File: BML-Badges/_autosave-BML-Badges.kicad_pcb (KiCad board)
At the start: 2 copper layers, 19 parts, among them Q1 PN2222A, Q2 PN2222A, Q3 PN2222A

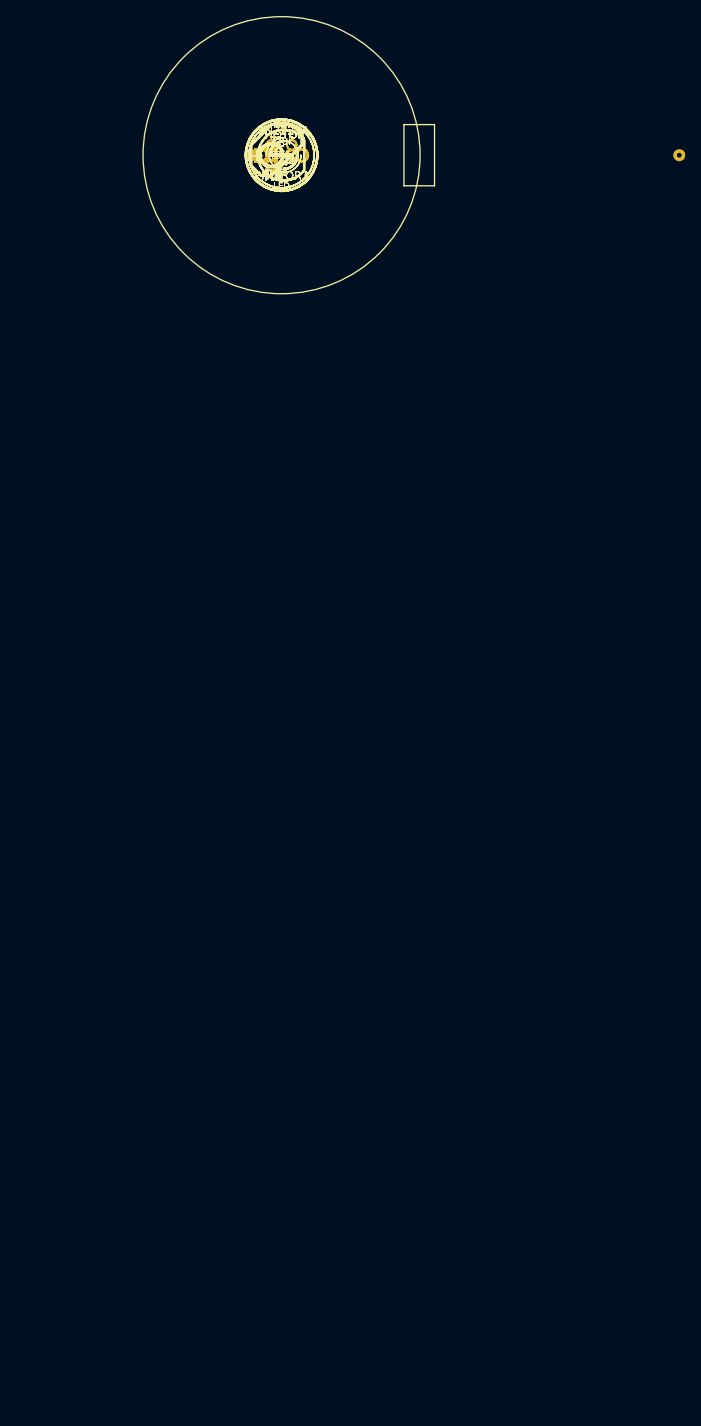
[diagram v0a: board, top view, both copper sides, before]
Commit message: Naptime
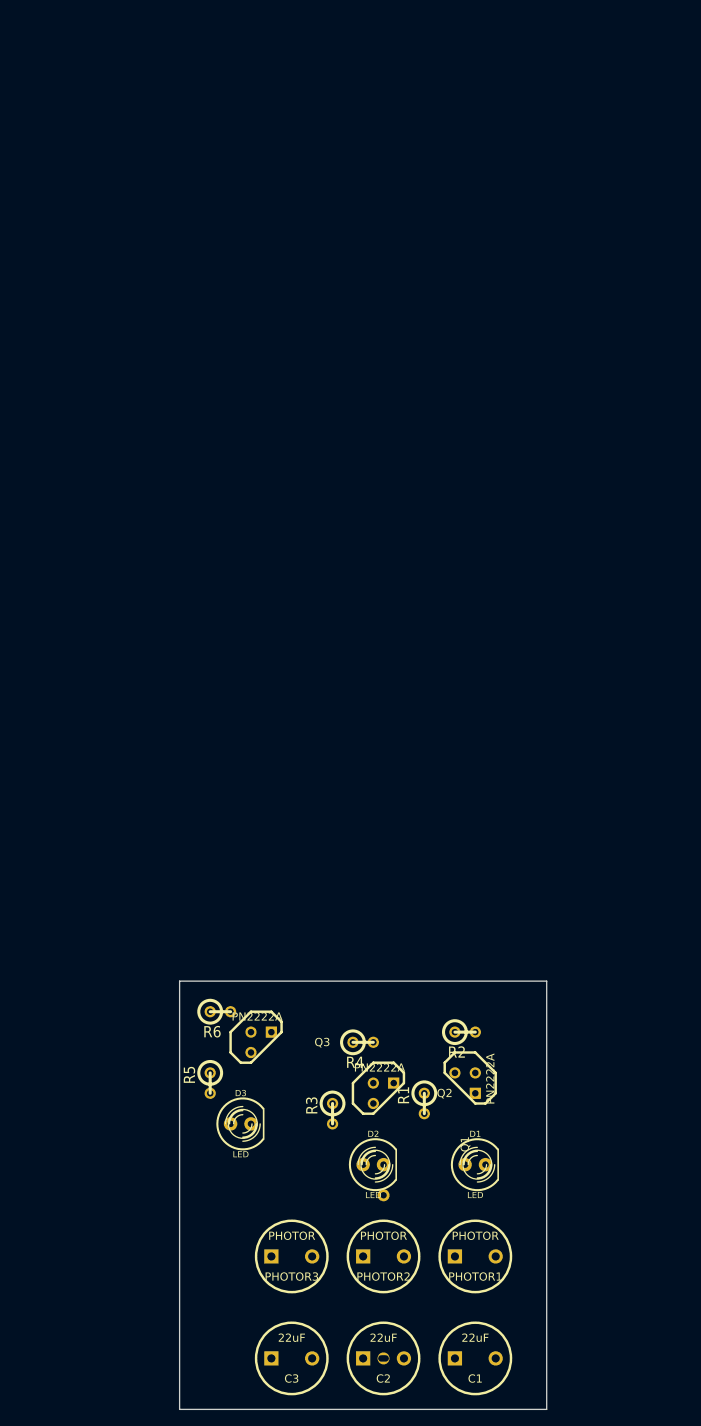
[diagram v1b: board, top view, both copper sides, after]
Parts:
- BT1: footprint BS-7 CR2032 -> BS-7-CR2032-2; moved to B.Cu
- C1, C2, C3: footprint C1V8 -> C2V8
- Q1, Q2, Q3: footprint TO92-CBE -> TO92-EBC-num
- moved C1 151.8 mm to (275.6, 232.4)
- moved C2 150.4 mm to (264.2, 232.4)
- moved C3 149.9 mm to (252.7, 232.4)
- moved PHOTOR1 139.3 mm to (275.6, 219.7)
- moved PHOTOR2 137.7 mm to (264.2, 219.7)
- moved PHOTOR3 137.2 mm to (252.7, 219.7)
- moved BT1 134.0 mm to (264.2, 215.9), turned to 270 degrees
- moved D1 128.0 mm to (275.6, 208.3)
- moved D2 126.2 mm to (262.9, 208.3)
- moved D3 120.8 mm to (246.4, 203.2)
- moved R3 119.5 mm to (257.8, 201.9), turned to 270 degrees
- moved R1 119.4 mm to (269.2, 200.7), turned to 270 degrees
- moved Q1 117.8 mm to (274.3, 198.1), turned to 270 degrees
- moved Q2 117.5 mm to (264.2, 199.4)
- moved R5 115.9 mm to (242.6, 198.1), turned to 270 degrees
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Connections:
- BT1 pad 2: N-000005 -> N-000008
- C1 pad 1: N-000004 -> N-000002
- C1 pad 2: N-000005 -> N-000008
- C2 pad 1: N-000003 (its old number) -> N-000009
- C2 pad 2: N-000005 -> N-000008
- C3 pad 1: N-000008 -> N-000006
- C3 pad 2: N-000005 -> N-000008
- D1 pad 2: N-000002 -> N-000001
- D2 pad 2: N-0000011 (its old number) -> N-000004
- D3 pad 2: N-000006 -> N-000005
- PHOTOR1 pad 1: N-000004 -> N-000002
- PHOTOR1 pad 2: N-000005 -> N-000008
- PHOTOR2 pad 1: N-000003 (its old number) -> N-000009
- PHOTOR2 pad 2: N-000005 -> N-000008
- PHOTOR3 pad 1: N-000008 -> N-000006
- PHOTOR3 pad 2: N-000005 -> N-000008
- R2 pad 2: N-000004 -> N-000002
- R4 pad 2: N-000003 (its old number) -> N-000009
- R6 pad 2: N-000008 -> N-000006
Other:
- board outline added: 45.7 x 53.3 mm

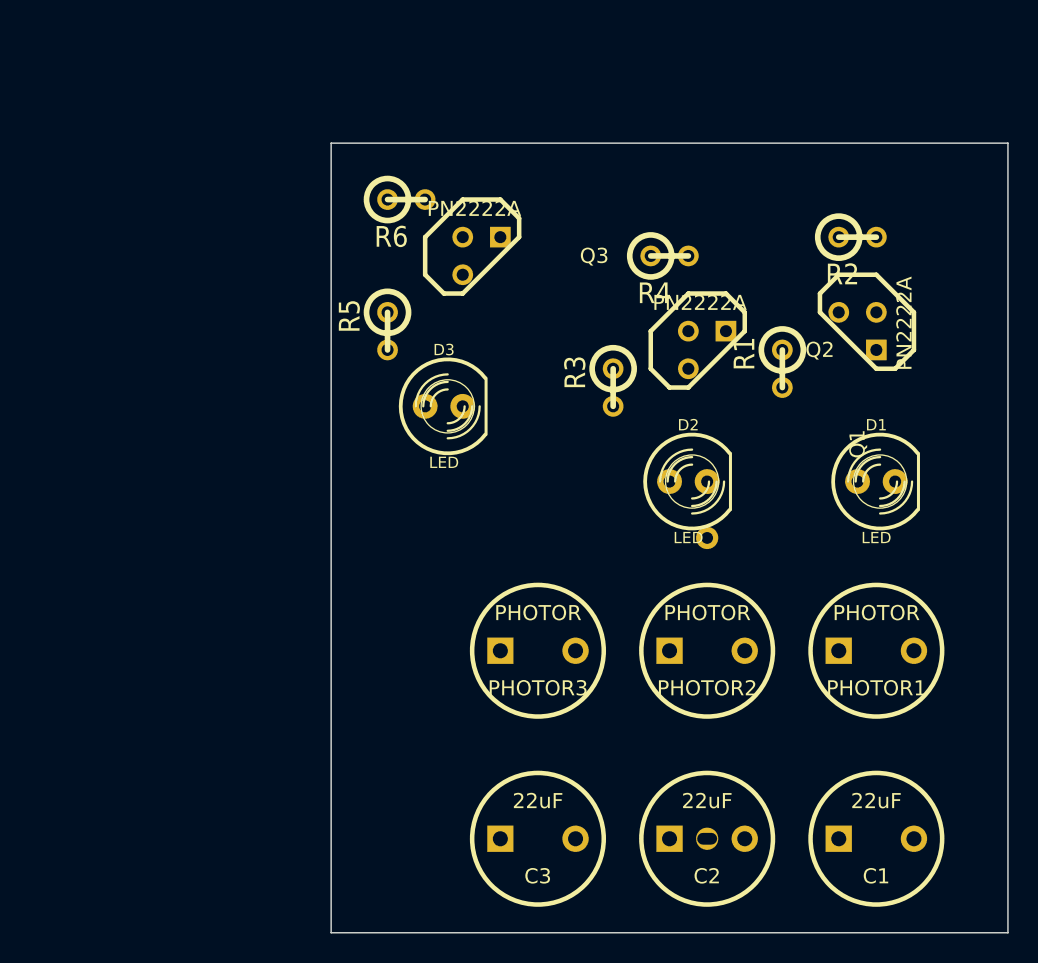
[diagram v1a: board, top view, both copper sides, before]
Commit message: version1complete
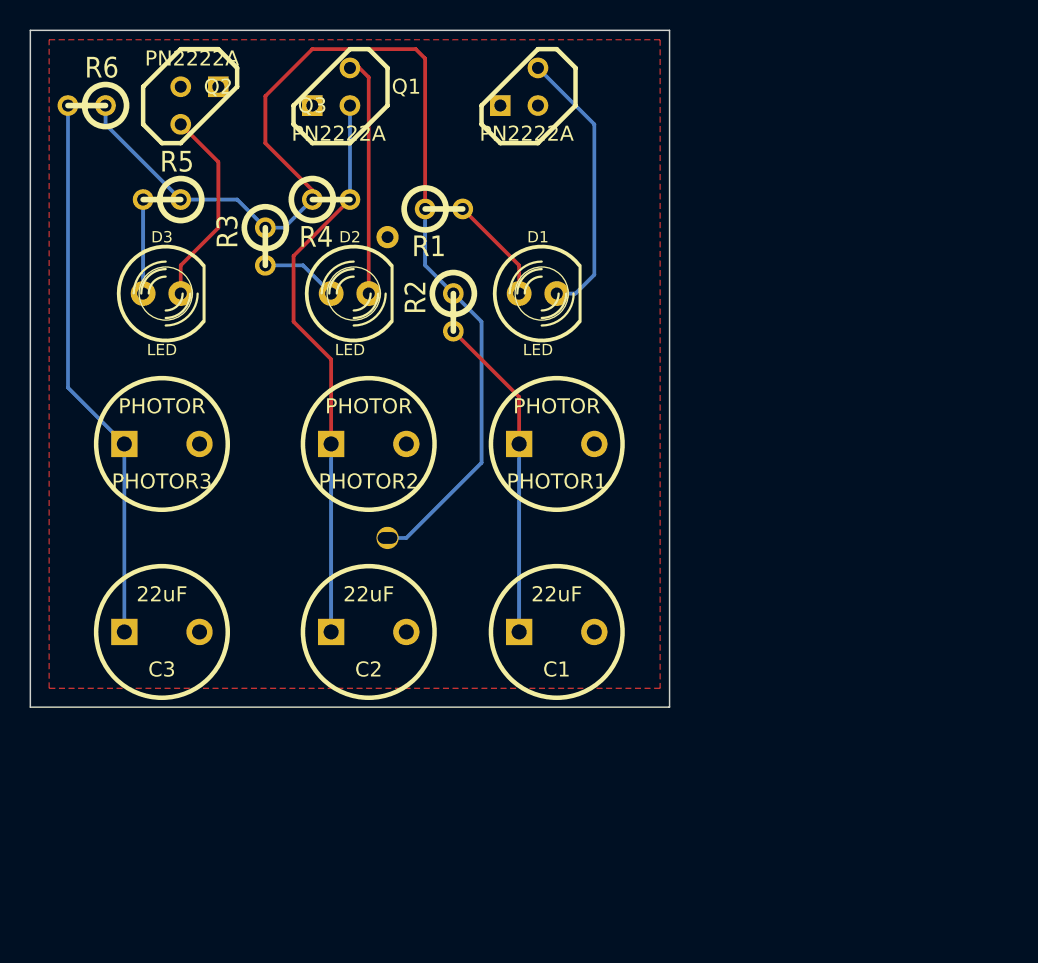
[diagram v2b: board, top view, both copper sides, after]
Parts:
- moved Q2 31.0 mm to (238.8, 181.6), turned to 180 degrees
- moved BT1 29.6 mm to (242.6, 195.6)
- moved C3 29.0 mm to (227.3, 218.4)
- moved PHOTOR3 29.0 mm to (227.3, 205.7)
- moved Q1 28.2 mm to (251.5, 181.6), turned to 180 degrees
- moved R2 27.8 mm to (247.0, 196.8), turned to 270 degrees
- moved C2 26.8 mm to (241.3, 218.4)
- moved PHOTOR2 26.8 mm to (241.3, 205.7)
- moved D1 26.2 mm to (252.7, 195.6)
- moved D2 26.2 mm to (240.0, 195.6)
- moved C1 25.7 mm to (254.0, 218.4)
- moved PHOTOR1 25.7 mm to (254.0, 205.7)
- moved R3 25.4 mm to (234.3, 192.4)
- moved R1 25.3 mm to (246.4, 189.9), turned to 0 degrees
- moved R4 23.2 mm to (238.8, 189.2)
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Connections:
- BT1 pad 2: N-000008 -> GND
- C1 pad 1: N-000002 (its old number) -> N-000001
- C1 pad 2: N-000008 -> GND
- C2 pad 2: N-000008 -> GND
- C3 pad 2: N-000008 -> GND
- PHOTOR1 pad 1: N-000002 (its old number) -> N-000001
- PHOTOR1 pad 2: N-000008 -> GND
- PHOTOR2 pad 2: N-000008 -> GND
- PHOTOR3 pad 2: N-000008 -> GND
- Q1 pad 1: N-000008 -> (no net)
- Q1 pad 2: N-000002 (its old number) -> GND
- Q2 pad 1: N-000008 -> (no net)
- Q3 pad 1: N-000008 -> (no net)
- Q3 pad 2: N-000006 -> GND
- R2 pad 2: N-000002 (its old number) -> N-000001
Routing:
- net N-0000010: track 0.00 -> 76.9 mm
- net N-000009: track 0.00 -> 38.2 mm
- net N-000006: track 0.00 -> 37.1 mm
- net N-000001: track 0.00 -> 22.2 mm
- net N-000002: track 0.00 -> 18.6 mm
- net N-000004: track 0.00 -> 16.1 mm
- net N-000005: track 0.00 -> 13.5 mm
- net N-000003: track 0.00 -> 7.29 mm
- net N-000007: track 0.00 -> 6.35 mm
- net N-0000011: track 0.00 -> 5.23 mm
- added copper zone on F.Cu, net GND
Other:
- board size 45.7 x 53.3 mm -> 43.2 x 45.7 mm
- board text added: "Karmanya Aggarwal BML Munjal University"
